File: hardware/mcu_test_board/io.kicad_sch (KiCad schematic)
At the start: 30 parts, among them CN7 KF2EDGR-2.54-9P, CN8 KF2EDGR-2.54-6P, U3 LTV-847S, U5 LTV-827S-TA1, U6 LTV-817S-TA1, U7 LTV-817S-TA1

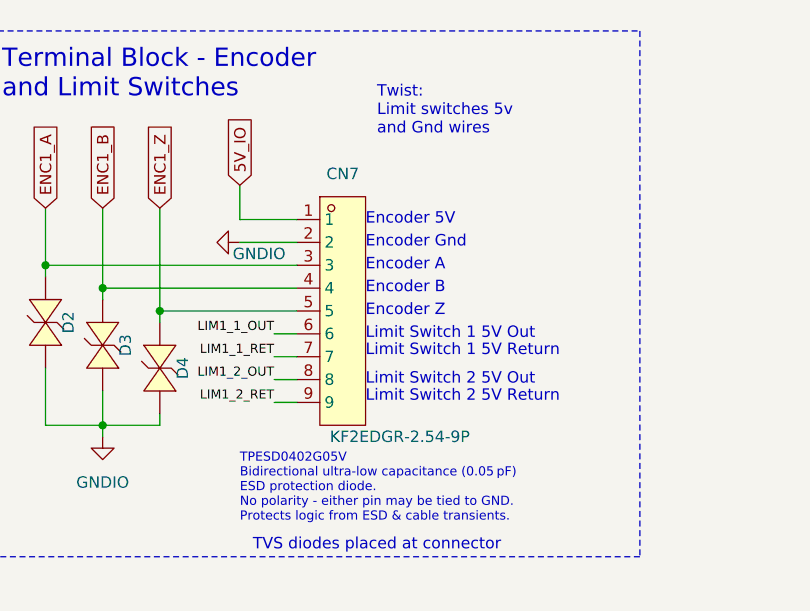
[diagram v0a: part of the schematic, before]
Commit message: Adjusting parts
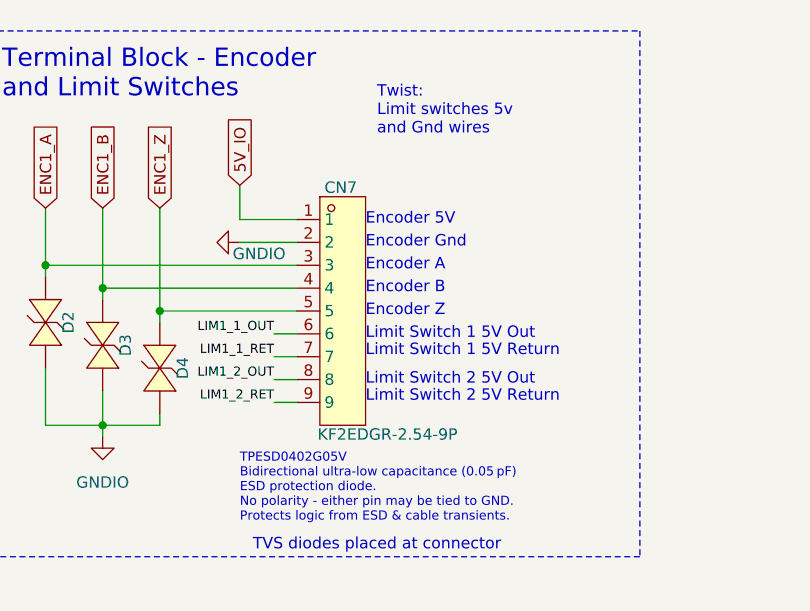
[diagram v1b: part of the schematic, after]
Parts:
- U5: footprint MyParts:LTV827S-TA1 -> MyParts:SMD-8_L9.8-W6.6-P2.54-LS10.3-BL
- U6, U7: footprint MyParts:LTV817S -> MyParts:OPTO-SMD-4_L4.6-W6.5-P2.54-LS10.3-BL
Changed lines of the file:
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@@
 	)
 	(symbol
-		(lib_name "TPESD0402G05V_4")
-		(lib_id "MyParts:TPESD0402G05V")
-		(at 167.64 69.85 270)
+		(lib_id "MyParts:KF2EDGR-2.54-9P")
+		(at 200.66 68.58 0)
 		(unit 1)
 		(exclude_from_sim no)
@@
 		(on_board yes)
 		(dnp no)
-		(property "Reference" "D2"
-			(at 170.18 69.85 0)
+		(property "Reference" "CN7"
+			(at 198.628 54.864 0)
 			(effects
 				(font
 					(size 1.27 1.27)
 				)
+				(justify left)
 			)
 		)
-		(property "Value" "TPESD0402G05V"
-			(at 162.56 69.85 0)
+		(property "Value" "KF2EDGR-2.54-9P"
+			(at 197.866 82.296 0)
 			(effects
 				(font
 					(size 1.27 1.27)
 				)
-				(hide yes)
+				(justify left)
 			)
 		)
-		(property "Footprint" "MyParts:D0402-BI"
-			(at 160.02 69.85 0)
+		(property "Footprint" "MyParts:CONN-TH_9P-P2.54_KF2EDGR-2.54-9P"
+			(at 200.66 86.36 0)
 			(effects
 				(font
@@
 			)
 		)
-		(property "Datasheet" ""
-			(at 167.64 69.85 0)
+		(property "Datasheet" "https://lcsc.com/product-detail/Pluggable-System-Terminal-Block_Cixi-Kefa-Elec-KF2EDGR-2-54-9P_C577601.html"
+			(at 200.66 88.9 0)
 			(effects
 				(font
@@
 		)
 		(property "Description" ""
-			(at 167.64 69.85 0)
+			(at 200.66 68.58 0)
 			(effects
 				(font
@@
 			)
 		)
-		(property "LCSC Part" "C558615"
-			(at 157.48 69.85 0)
+		(property "LCSC Part" "C577601"
+			(at 200.66 91.44 0)
 			(effects
 				(font
@@
 			)
 		)
+		(pin "1"
+		)
+		(pin "5"
+		)
+		(pin "8"
+		)
+		(pin "6"
+		)
+		(pin "7"
+		)
 		(pin "2"
 		)
-		(pin "1"
+		(pin "9"
+		)
+		(pin "3"
+		)
+		(pin "4"
 		)
 		(instances
-			(project "mcu_test_board"
+			(project ""
 				(path "/262d8f76-cfc1-4cac-8f67-8c56cd47dd59/3ab438cf-211a-4f77-8c57-80f47d57ba40"
-					(reference "D2")
+					(reference "CN7")
 					(unit 1)
 				)
@@
 	)
 	(symbol
-		(lib_id "MyParts:LTV-847S")
-		(at 78.74 67.31 0)
+		(lib_name "TPESD0402G05V_4")
+		(lib_id "MyParts:TPESD0402G05V")
+		(at 167.64 69.85 270)
 		(unit 1)
 		(exclude_from_sim no)
@@
 		(on_board yes)
 		(dnp no)
-		(fields_autoplaced yes)
-		(property "Reference" "U3"
-			(at 78.74 46.99 0)
+		(property "Reference" "D2"
+			(at 170.18 69.85 0)
 			(effects
 				(font
@@
 			)
 		)
-		(property "Value" "LTV-847S"
-			(at 78.74 49.53 0)
+		(property "Value" "TPESD0402G05V"
+			(at 162.56 69.85 0)
 			(effects
 				(font
 					(size 1.27 1.27)
 				)
+				(hide yes)
 			)
 		)
-		(property "Footprint" "MyParts:SMD-16_L20.0-W6.5-P2.54-LS10.2-BL"
-			(at 78.74 88.9 0)
+		(property "Footprint" "MyParts:D0402-BI"
+			(at 160.02 69.85 0)
 			(effects
 				(font
@@
 			)
 		)
-		(property "Datasheet" "https://lcsc.com/product-detail/SMD-Optocouplers_LTV-847S_C114599.html"
-			(at 78.74 91.44 0)
+		(property "Datasheet" ""
+			(at 167.64 69.85 0)
 			(effects
 				(font
@@
 		)
 		(property "Description" ""
-			(at 78.74 67.31 0)
+			(at 167.64 69.85 0)
 			(effects
 				(font
@@
 			)
 		)
-		(property "LCSC Part" "C114599"
-			(at 78.74 93.98 0)
+		(property "LCSC Part" "C558615"
+			(at 157.48 69.85 0)
 			(effects
 				(font
@@
 			)
 		)
-		(pin "7"
-		)
-		(pin "16"
-		)
-		(pin "9"
-		)
-		(pin "3"
-		)
-		(pin "5"
-		)
-		(pin "4"
-		)
 		(pin "2"
 		)
-		(pin "6"
-		)
 		(pin "1"
 		)
-		(pin "8"
-		)
-		(pin "10"
-		)
-		(pin "14"
-		)
-		(pin "12"
-		)
-		(pin "11"
-		)
-		(pin "15"
-		)
-		(pin "13"
-		)
 		(instances
 			(project "mcu_test_board"
 				(path "/262d8f76-cfc1-4cac-8f67-8c56cd47dd59/3ab438cf-211a-4f77-8c57-80f47d57ba40"
-					(reference "U3")
+					(reference "D2")
 					(unit 1)
 				)
@@
 	)
 	(symbol
+		(lib_id "MyParts:LTV-847S")
+		(at 78.74 67.31 0)
+		(unit 1)
+		(exclude_from_sim no)
+		(in_bom yes)
+		(on_board yes)
+		(dnp no)
+		(fields_autoplaced yes)
+		(property "Reference" "U3"
+			(at 78.74 46.99 0)
+			(effects
+				(font
+					(size 1.27 1.27)
+				)
+			)
+		)
+		(property "Value" "LTV-847S"
+			(at 78.74 49.53 0)
+			(effects
+				(font
+					(size 1.27 1.27)
+				)
+			)
+		)
+		(property "Footprint" "MyParts:SMD-16_L20.0-W6.5-P2.54-LS10.2-BL"
+			(at 78.74 88.9 0)
+			(effects
+				(font
+					(size 1.27 1.27)
+				)
+				(hide yes)
+			)
+		)
+		(property "Datasheet" "https://lcsc.com/product-detail/SMD-Optocouplers_LTV-847S_C114599.html"
+			(at 78.74 91.44 0)
+			(effects
+				(font
+					(size 1.27 1.27)
+				)
+				(hide yes)
+			)
+		)
+		(property "Description" ""
+			(at 78.74 67.31 0)
+			(effects
+				(font
+					(size 1.27 1.27)
+				)
+				(hide yes)
+			)
+		)
+		(property "LCSC Part" "C114599"
+			(at 78.74 93.98 0)
+			(effects
+				(font
+					(size 1.27 1.27)
+				)
+				(hide yes)
+			)
+		)
+		(pin "7"
+		)
+		(pin "6"
+		)
+		(pin "5"
+		)
+		(pin "8"
+		)
+		(pin "14"
+		)
+		(pin "16"
+		)
+		(pin "2"
+		)
+		(pin "1"
+		)
+		(pin "4"
+		)
+		(pin "3"
+		)
+		(pin "13"
+		)
+		(pin "15"
+		)
+		(pin "12"
+		)
+		(pin "10"
+		)
+		(pin "9"
+		)
+		(pin "11"
+		)
+		(instances
+			(project ""
+				(path "/262d8f76-cfc1-4cac-8f67-8c56cd47dd59/3ab438cf-211a-4f77-8c57-80f47d57ba40"
+					(reference "U3")
+					(unit 1)
+				)
+			)
+		)
+	)
+	(symbol
 		(lib_id "PCM_JLCPCB-Resistors:0402,470Ω")
 		(at 54.61 130.81 90)
@@
 			)
 		)
-		(property "Footprint" "MyParts:LTV827S-TA1"
+		(property "Footprint" "MyParts:SMD-8_L9.8-W6.6-P2.54-LS10.3-BL"
 			(at 77.47 151.13 0)
 			(effects
@@
 	)
 	(symbol
-		(lib_id "MyParts:KF2EDGR-2.54-9P")
-		(at 200.66 68.58 0)
-		(unit 1)
-		(exclude_from_sim no)
-		(in_bom yes)
-		(on_board yes)
-		(dnp no)
-		(property "Reference" "CN7"
-			(at 200.66 53.34 0)
-			(effects
-				(font
-					(size 1.27 1.27)
-				)
-			)
-		)
-		(property "Value" "KF2EDGR-2.54-9P"
-			(at 207.01 82.55 0)
-			(effects
-				(font
-					(size 1.27 1.27)
-				)
-			)
-		)
-		(property "Footprint" "MyParts:CONN-TH_9P-P2.54_KF2EDGR-2.54-9P"
-			(at 200.66 86.36 0)
-			(effects
-				(font
-					(size 1.27 1.27)
-				)
-				(hide yes)
-			)
-		)
-		(property "Datasheet" "https://lcsc.com/product-detail/Pluggable-System-Terminal-Block_Cixi-Kefa-Elec-KF2EDGR-2-54-9P_C577601.html"
-			(at 200.66 88.9 0)
-			(effects
-				(font
-					(size 1.27 1.27)
-				)
-				(hide yes)
-			)
-		)
-		(property "Description" ""
-			(at 200.66 68.58 0)
-			(effects
-				(font
-					(size 1.27 1.27)
-				)
-				(hide yes)
-			)
-		)
-		(property "LCSC Part" "C577601"
-			(at 200.66 91.44 0)
-			(effects
-				(font
-					(size 1.27 1.27)
-				)
-				(hide yes)
-			)
-		)
-		(pin "3"
-		)
-		(pin "5"
-		)
-		(pin "6"
-		)
-		(pin "8"
-		)
-		(pin "1"
-		)
-		(pin "7"
-		)
-		(pin "2"
-		)
-		(pin "4"
-		)
-		(pin "9"
-		)
-		(instances
-			(project "mcu_test_board"
-				(path "/262d8f76-cfc1-4cac-8f67-8c56cd47dd59/3ab438cf-211a-4f77-8c57-80f47d57ba40"
-					(reference "CN7")
-					(unit 1)
-				)
-			)
-		)
-	)
-	(symbol
 		(lib_id "MyParts:LTV-817S-TA1")
 		(at 77.47 153.67 0)
@@
 			)
 		)
-		(property "Footprint" "MyParts:LTV817S"
+		(property "Footprint" "MyParts:OPTO-SMD-4_L4.6-W6.5-P2.54-LS10.3-BL"
 			(at 77.47 163.83 0)
 			(effects
@@
 	)
 	(symbol
+		(lib_name "LTV-817S-TA1_1")
 		(lib_id "MyParts:LTV-817S-TA1")
 		(at 77.47 166.37 0)
@@
 			)
 		)
-		(property "Footprint" "MyParts:LTV817S"
+		(property "Footprint" "MyParts:OPTO-SMD-4_L4.6-W6.5-P2.54-LS10.3-BL"
 			(at 77.47 176.53 0)
 			(effects
